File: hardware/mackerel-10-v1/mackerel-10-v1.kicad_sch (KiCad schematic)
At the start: 4 parts, among them J1 Conn_02x05_Odd_Even, U1 68010D, X1 40 MHz

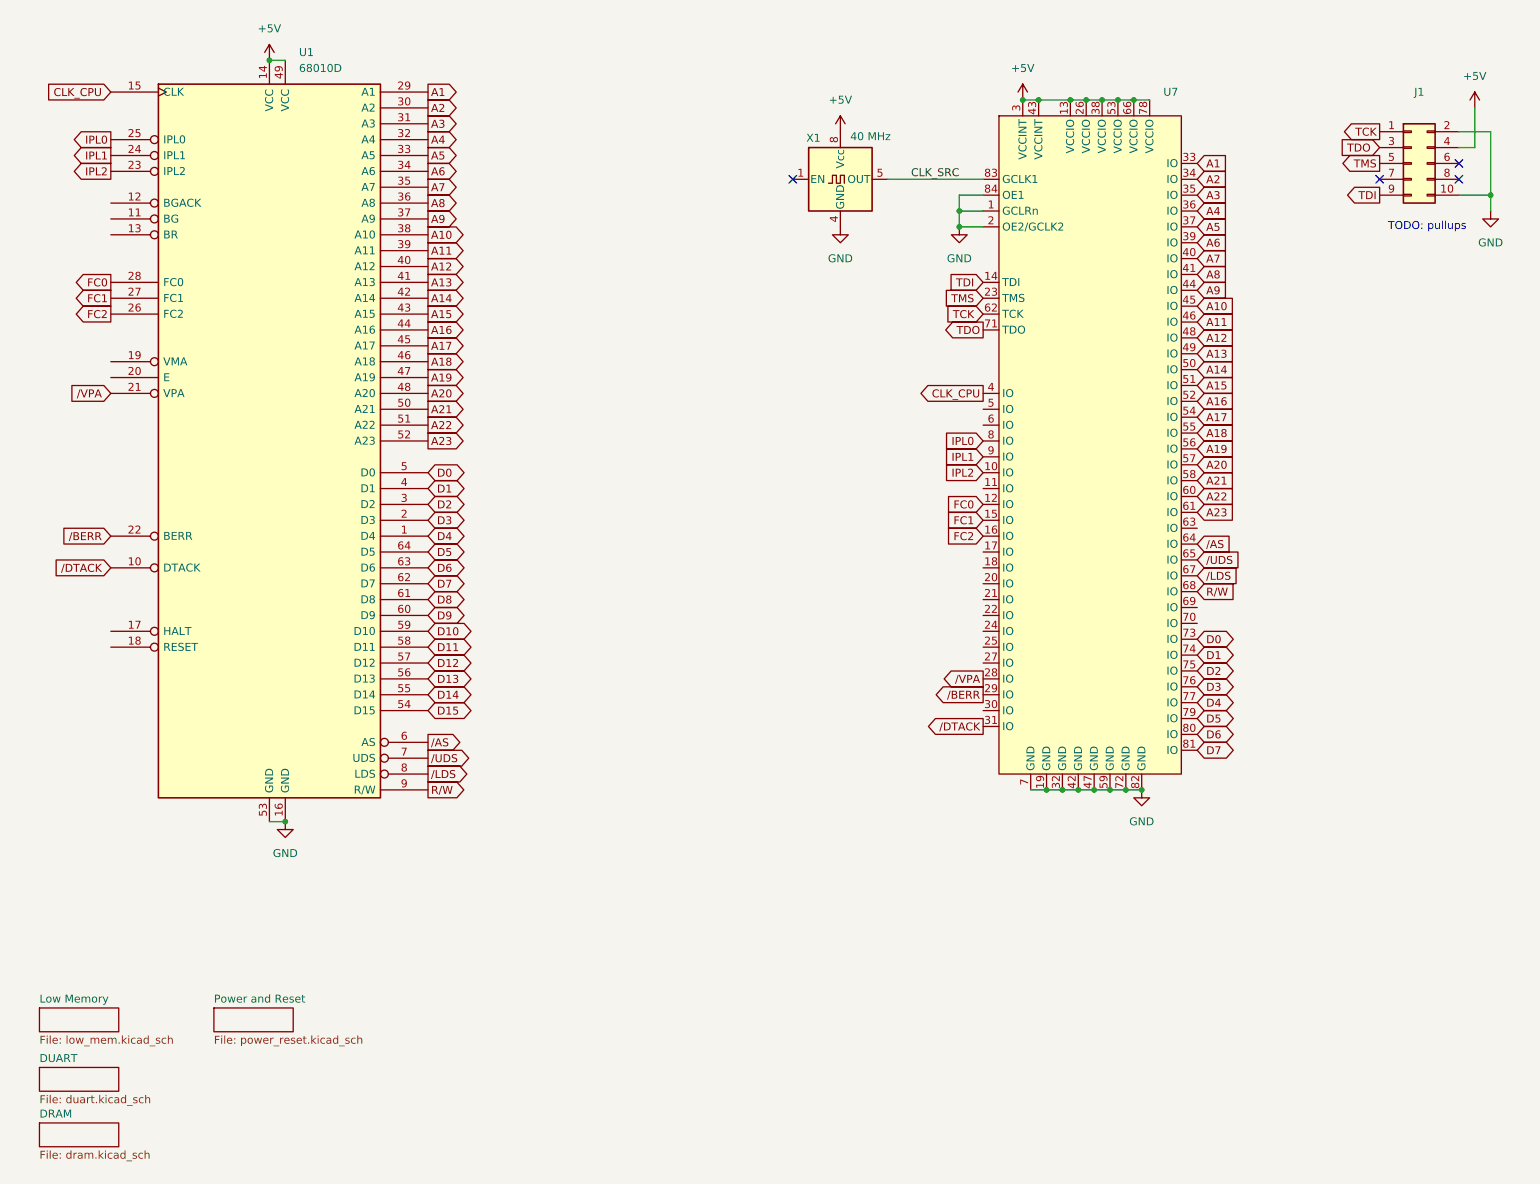
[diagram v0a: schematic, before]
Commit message: Trying to figure out Mackerel-10 components
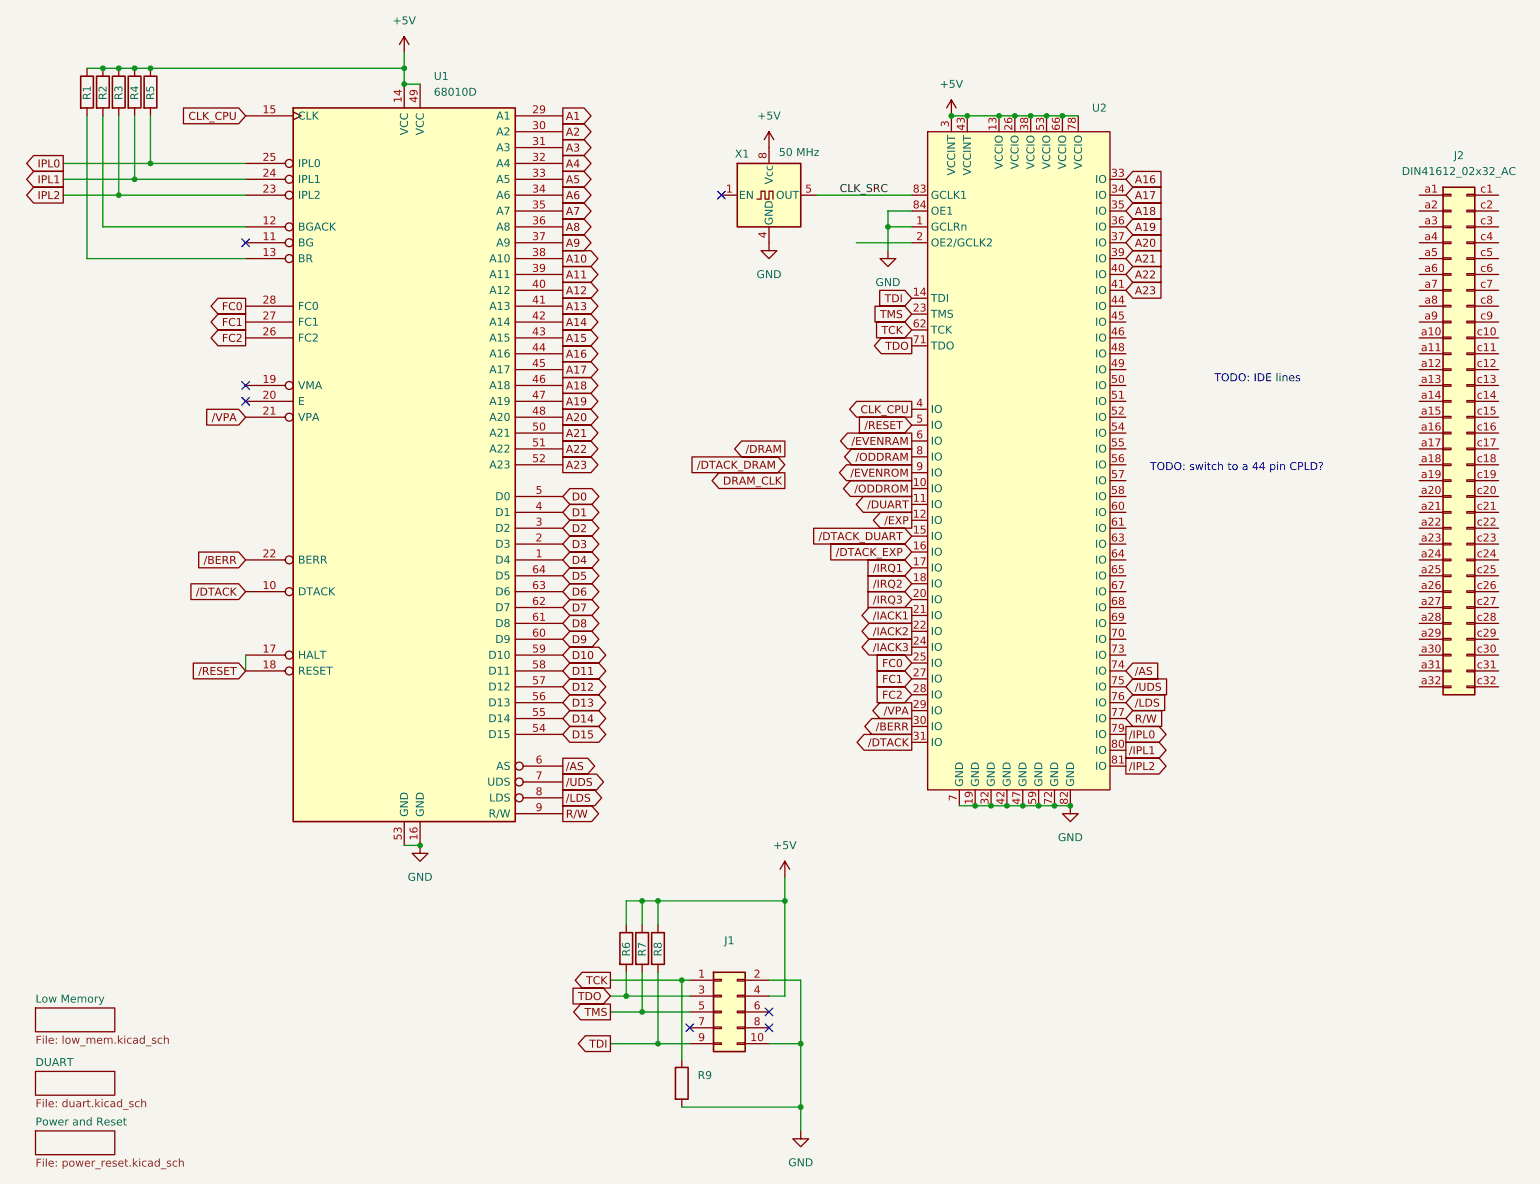
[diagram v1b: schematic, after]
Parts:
- added J2: DIN41612_02x32_AC, Connector_DIN:DIN41612_C_2x32_Male_Horizontal_THT, symbol Connector:DIN41612_02x32_AC
- added R1, R2, R3, R4, R5, R6, R7, R8, R9: R, Resistor_THT:R_Axial_DIN0204_L3.6mm_D1.6mm_P5.08mm_Horizontal, symbol Device:R
- X1: value 40 MHz -> 50 MHz
- renumbered U7 to U2
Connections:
- net +5V: now also R1.1, R2.1, R3.1, R4.1, R5.1, R6.1, R7.1, R8.1
- net A1: no longer U2.33 (IO)
- net A10: no longer U2.45 (IO)
- net A11: no longer U2.46 (IO)
- net A12: no longer U2.48 (IO)
- net A13: no longer U2.49 (IO)
- net A14: no longer U2.50 (IO)
- net A15: no longer U2.51 (IO)
- net A16: now also U2.33 (IO); no longer U2.52 (IO)
- net A17: now also U2.34 (IO); no longer U2.54 (IO)
- net A18: now also U2.35 (IO); no longer U2.55 (IO)
- net A19: now also U2.36 (IO); no longer U2.56 (IO)
- net A2: no longer U2.34 (IO)
- net A20: now also U2.37 (IO); no longer U2.57 (IO)
- net A21: now also U2.39 (IO); no longer U2.58 (IO)
- net A22: now also U2.40 (IO); no longer U2.60 (IO)
- net A23: now also U2.41 (IO); no longer U2.61 (IO)
- net A3: no longer U2.35 (IO)
- net A4: no longer U2.36 (IO)
- net A5: no longer U2.37 (IO)
- net A6: no longer U2.39 (IO)
- net A7: no longer U2.40 (IO)
- net A8: no longer U2.41 (IO)
- net A9: no longer U2.44 (IO)
- net D0: no longer U2.73 (IO)
- net D1: no longer U2.74 (IO)
- net D2: no longer U2.75 (IO)
- net D3: no longer U2.76 (IO)
- net D4: no longer U2.77 (IO)
- net D5: no longer U2.79 (IO)
- net D6: no longer U2.80 (IO)
- net D7: no longer U2.81 (IO)
- net FC0: now also U2.25 (IO); no longer U2.12 (IO)
- net FC1: now also U2.27 (IO); no longer U2.15 (IO)
- net FC2: now also U2.28 (IO); no longer U2.16 (IO)
- net GND: now also R9.2; no longer U2.2 (OE2/GCLK2)
- net IPL0: now also R5.2; no longer U2.8 (IO)
- net IPL1: now also R4.2; no longer U2.9 (IO)
- net IPL2: now also R3.2; no longer U2.10 (IO)
- net R/W: now also U2.77 (IO); no longer U2.68 (IO)
- net TCK: now also R9.1
- net TDI: now also R8.2
- net TDO: now also R6.2
- net TMS: now also R7.2
- net /AS: now also U2.74 (IO); no longer U2.64 (IO)
- net /BERR: now also U2.30 (IO); no longer U2.29 (IO)
- net /LDS: now also U2.76 (IO); no longer U2.67 (IO)
- net /UDS: now also U2.75 (IO); no longer U2.65 (IO)
- net /VPA: now also U2.29 (IO); no longer U2.28 (IO)
- net at U1.12 (BGACK): now also R2.2
- net at U1.13 (BR): now also R1.2
- net /RESET: now reaches U1.17 (HALT)
- net /RESET: now also U1.18 (RESET), U2.5 (IO)
- net /DUART: now reaches U2.11 (IO)
- net /IRQ1: now reaches U2.17 (IO)
- net /IRQ2: now reaches U2.18 (IO)
- net /IRQ3: now reaches U2.20 (IO)
- net /IACK1: now reaches U2.21 (IO)
- net /IACK2: now reaches U2.22 (IO)
- net /IACK3: now reaches U2.24 (IO)
- net /EVENRAM: now reaches U2.6 (IO)
- new net /DTACK_DUART: U2.15 (IO)
- new net /DTACK_EXP: U2.16 (IO)
- new net /EVENROM: U2.9 (IO)
- new net /EXP: U2.12 (IO)
- new net /IPL0: U2.79 (IO)
- new net /IPL1: U2.80 (IO)
- new net /IPL2: U2.81 (IO)
- new net /ODDRAM: U2.8 (IO)
- new net /ODDROM: U2.10 (IO)
- no-connect marks 4 -> 7
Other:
- removed sheet DRAM
- note added: "TODO: IDE lines"
- note added: "TODO: switch to a 44 pin CPLD?"
- note removed: "TODO: pullups"
- moved on the sheet: J1, U1, U2, X1
